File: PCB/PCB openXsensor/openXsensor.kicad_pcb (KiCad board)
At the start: 2 copper layers, 32.4 x 33 mm, 33 parts, among them P1 Digital, P10 VFAS/COURANT, P11 GY-86, P12 NTC1, P13 NTC2, P14 ALIM, P15 STRAP, P16 4S, P17 ADS1115, P18 ADS_IN, P2 Analog, P3 ADC, P4 ADC, P4-2 ADC, P5 GPS, P6 HUB/SPORT, P7 PPM, P8 FUEL, P9 RPM

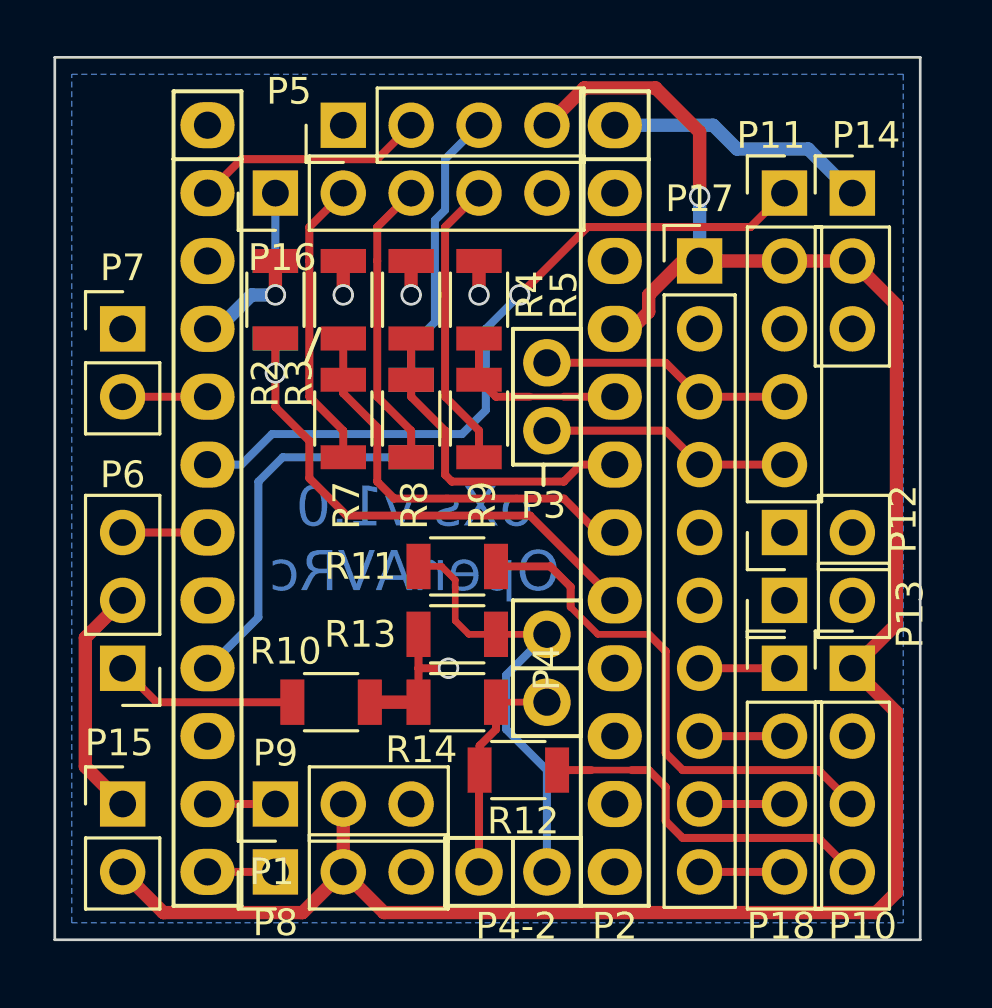
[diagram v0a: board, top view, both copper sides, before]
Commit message: Update oXs pcb
Add sequencer connector
Add capacitors on analog input 
Add capacitors on 5v and raw power 
...
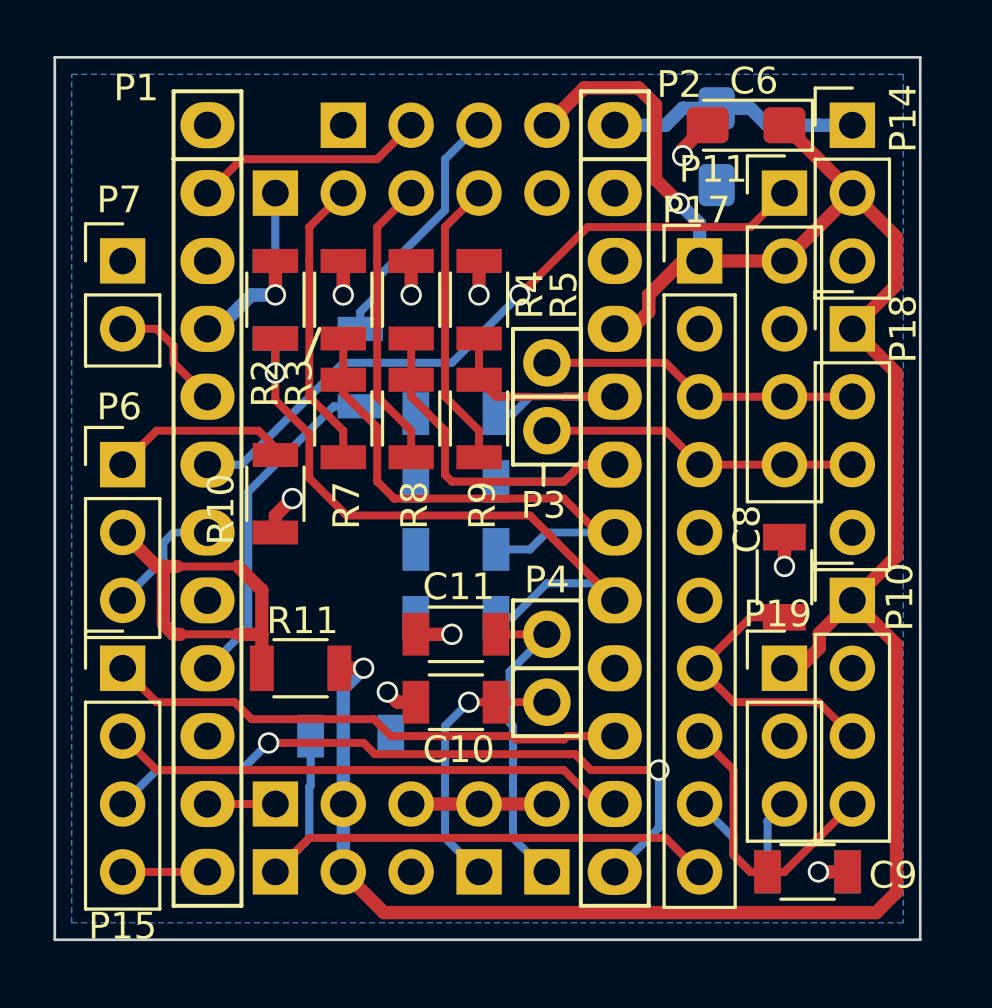
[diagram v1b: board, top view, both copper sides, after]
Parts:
- removed P4-2: ADC, Socket_Arduino_Pro_Mini:Socket_Strip_Arduino_1x02
- removed R12: 51K, R_1206
- removed R13, R14: 20K, R_1206
- added C1: 100nF, Empreintes:C_1206, B.Cu at (147.7, 103.5)
- added C10: 100nF, Empreintes:C_1206, F.Cu at (147.7, 106.7)
- added C11: 100nF, Empreintes:C_1206, F.Cu at (147.7, 104.1)
- added C14: 100nF, Empreintes:C_1206, B.Cu at (143.8, 108.0)
- added C2: 100nF, Empreintes:C_1206, B.Cu at (147.7, 101.0)
- added C3: 100nF, Empreintes:C_1206, B.Cu at (147.7, 98.4)
- added C4: 100nF, Empreintes:C_1206, B.Cu at (147.7, 95.9)
- added C5: 10uF, Empreintes:CP_EIA-3216-18_Kemet-A_Pad1.58x1.35mm_HandSolder, B.Cu at (157.5, 85.9)
- added C6: 10uF, Empreintes:CP_EIA-3216-18_Kemet-A_Pad1.58x1.35mm_HandSolder, F.Cu at (158.6, 85.1)
- added C7: 100nF, Empreintes:C_1206, B.Cu at (160.9, 113.0)
- added C8: 100nF, Empreintes:C_1206, F.Cu at (160.0, 102.0)
- added C9: 100nF, Empreintes:C_1206, F.Cu at (160.9, 113.0)
- added P19: MPXV7002DP, Pin_Header_Straight_1x03_Pitch2.54mm, F.Cu at (160.0, 105.4)
- P12, P13, P16, P5, P8, P9: moved to B.Cu
- P15: value STRAP -> SEQUENCEUR; footprint Pin_Header_Straight_1x02_Pitch2.54mm -> Pin_Header_Straight_1x04_Pitch2.54mm
- P18: value ADS_IN -> MS4525DO
- R11: value 51K -> 0
- moved P12 17.1 mm to (148.6, 113.0), turned to 0 degrees
- moved P13 13.5 mm to (151.1, 113.0), turned to 0 degrees
- moved P18 13.0 mm to (162.6, 92.7)
- moved R10 8.07 mm to (141.0, 98.9), turned to 270 degrees
- moved P6 7.62 mm to (135.3, 97.8), turned to 0 degrees
- moved R11 6.99 mm to (141.9, 105.4), turned to 0 degrees
- moved P15 5.08 mm to (135.3, 105.4)
- moved R1 2.69 mm to (144.1, 94.2)
- moved P10 2.54 mm to (162.6, 102.9)
- moved P14 2.54 mm to (162.6, 85.1)
- moved P7 2.54 mm to (135.3, 90.2)
- turned P16 to 270 degrees
- turned P5 to 270 degrees
- turned P8 to 270 degrees
- turned P9 to 270 degrees
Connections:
- P1 pad 12: /9(**) -> /SEQ1
- P10 pad 3: Net-(P10-Pad3) -> /ADS_VOLT1
- P10 pad 4: Net-(P10-Pad4) -> /ADS_VOLT2
- P12 pad 1: (no net) -> /A6
- P13 pad 1: (no net) -> /A7
- P15 pad 1: Net-(P15-Pad1) -> /SEQ4
- P15 pad 2: VCC -> /SEQ3
- P17 pad 10: Net-(P17-Pad10) -> /ADS_VOLT4
- P17 pad 7: Net-(P17-Pad7) -> /ADS_VOLT1
- P17 pad 8: Net-(P17-Pad8) -> /ADS_VOLT2
- P17 pad 9: Net-(P17-Pad9) -> /ADS_VOLT3
- P18 pad 1: Net-(P17-Pad7) -> VCC
- P18 pad 2: Net-(P17-Pad8) -> /A5
- P18 pad 3: Net-(P17-Pad9) -> /A4
- P18 pad 4: Net-(P17-Pad10) -> GND
- P2 pad 10: (no net) -> /SEQ4
- P2 pad 11: (no net) -> /SEQ3
- P2 pad 12: (no net) -> /SEQ2
- P6 pad 2: Net-(P15-Pad1) -> Net-(P6-Pad2)
- P8 pad 1: /9(**) -> /ADS_VOLT4
- R11 pad 1: Net-(P10-Pad3) -> Net-(P6-Pad2)
- R11 pad 2: /A7 -> VCC
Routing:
- net /SEQ2: track 0.00 -> 25.9 mm, vias 0 -> 2
- net /ADS_VOLT4: track 0.00 -> 22.6 mm
- net Net-(P10-Pad3): track 19.7 -> 0.00 mm
- net /SEQ4: track 0.00 -> 19.6 mm
- net /SEQ3: track 0.00 -> 19.5 mm
- net Net-(P6-Pad2): track 0.00 -> 15.0 mm
- net Net-(P10-Pad4): track 13.4 -> 0.00 mm
- net /ADS_VOLT1: track 0.00 -> 10.7 mm
- net /ADS_VOLT2: track 0.00 -> 10.7 mm
- net VCC: track 81.5 -> 90.4 mm, vias 1 -> 2
- net Net-(P15-Pad1): track 8.78 -> 0.00 mm
- net GND: track 13.6 -> 21.6 mm, vias 5 -> 10
- net /ADS_VOLT3: track 0.00 -> 6.77 mm
- net /A0: track 20.4 -> 25.6 mm
- net /A7: track 16.9 -> 12.0 mm
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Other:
- board text added: "OpenAVRc oXs v1.0"
- board text removed: "oXs v1.0 OpenAVRc"
